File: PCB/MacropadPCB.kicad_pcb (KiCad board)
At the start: 2 copper layers, 38.3 x 79.7 mm, 9 parts, among them SW1 SW_Push, SW2 SW_Push, SW3 SW_Push, SW4 SW_Push, SW5 SW_Push, SW6 SW_Push, U1 XIAO-RP2040-DIP

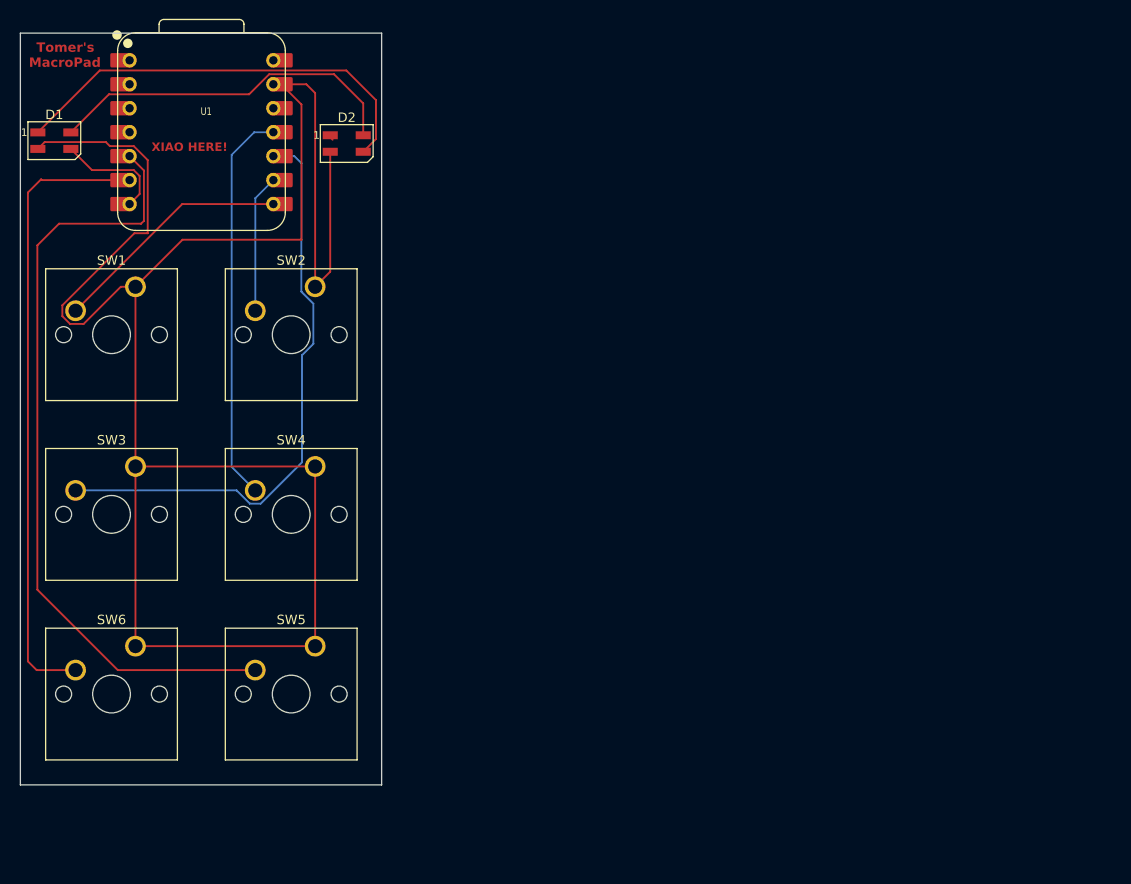
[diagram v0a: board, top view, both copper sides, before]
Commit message: VERSION 3
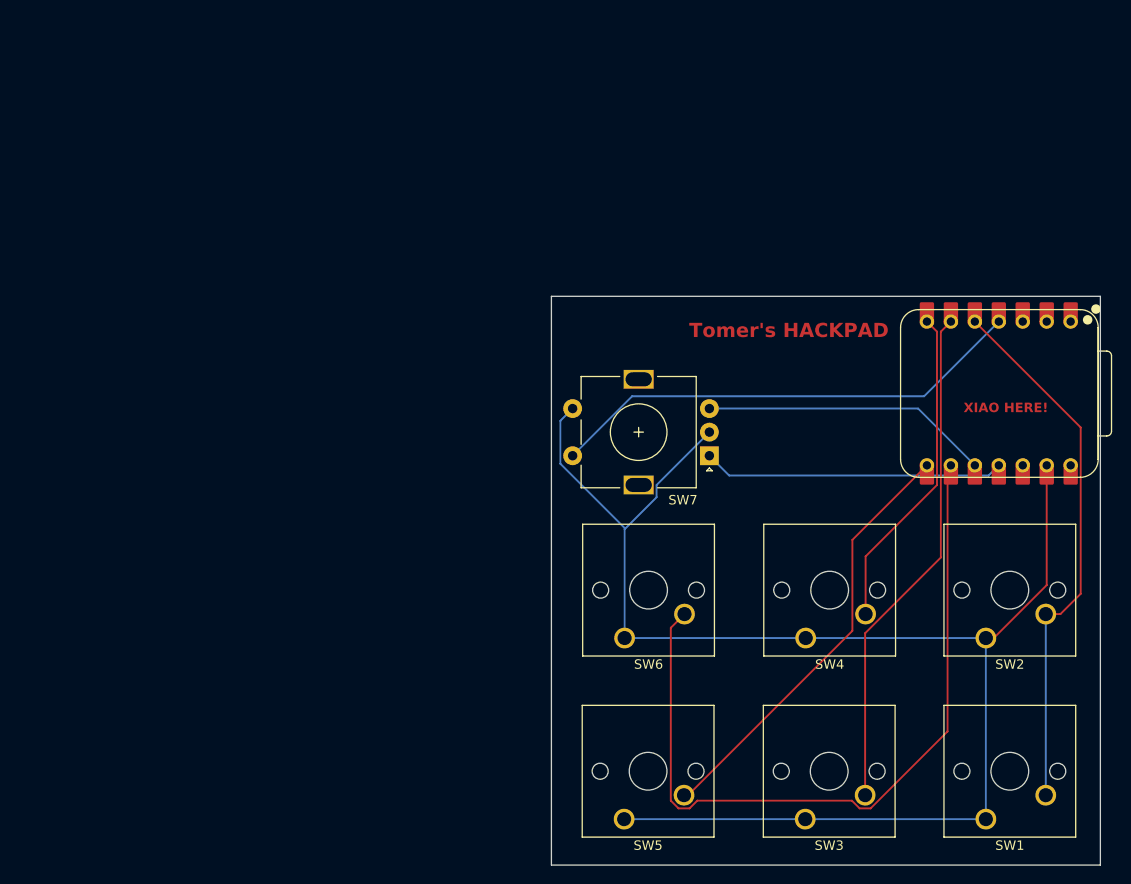
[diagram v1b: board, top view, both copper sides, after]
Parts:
- removed D1, D2: SK6812MINI, LED_SMD:LED_SK6812MINI_PLCC4_3.5x3.5mm_P1.75mm
- added SW7: RotaryEncoder_Switch, Rotary_Encoder:RotaryEncoder_Alps_EC11E-Switch_Vertical_H20mm, F.Cu at (144.3, 105.7)
- moved SW1 106.4 mm to (173.7, 144.2), turned to 180 degrees
- moved U1 89.0 mm to (175.0, 99.1), turned to -90 degrees
- moved SW2 80.3 mm to (173.7, 125.0), turned to 180 degrees
- moved SW3 80.3 mm to (154.5, 144.2), turned to 180 degrees
- moved SW4 55.1 mm to (154.6, 125.0), turned to 180 degrees
- moved SW6 51.9 mm to (135.4, 125.0), turned to 180 degrees
- moved SW5 37.5 mm to (135.3, 144.2), turned to 180 degrees
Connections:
- SW1 pad 2: Net-(U1-GPIO1/RX) -> Net-(U1-GPIO6/SDA)
- SW2 pad 2: Net-(U1-GPIO2/SCK) -> Net-(U1-GPIO6/SDA)
- SW3 pad 2: Net-(U1-GPIO4/MISO) -> Net-(U1-GPIO7/SCL)
- SW4 pad 2: Net-(U1-GPIO3/MOSI) -> Net-(U1-GPIO0/TX)
- SW5 pad 2: Net-(U1-GPIO6/SDA) -> Net-(U1-GPIO1/RX)
- SW6 pad 2: Net-(U1-GPIO7/SCL) -> Net-(U1-GPIO2/SCK)
- U1 pad 4: unconnected-(U1-GPIO29/ADC3/A3-Pad4) -> Net-(U1-GPIO29/ADC3/A3)
- U1 pad 7: Net-(D1-DIN) -> Net-(U1-GPIO0/TX)
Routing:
- net Net-(U1-GPIO2/SCK): track 14.6 -> 82.5 mm
- net GND: track 216.2 -> 158.2 mm
- net Net-(U1-GPIO29/ADC3/A3): track 0.00 -> 51.1 mm
- net Net-(D1-DOUT): track 45.9 -> 0.00 mm
- net Net-(D1-VDD): track 38.2 -> 0.00 mm
- net Net-(U1-GPIO0/TX): track 0.00 -> 34.6 mm
- net Net-(U1-GPIO4/MISO): track 62.4 -> 30.6 mm
- net Net-(U1-GPIO6/SDA): track 83.0 -> 57.3 mm
- net Net-(U1-GPIO1/RX): track 25.7 -> 45.9 mm
- net Net-(D1-DIN): track 11.9 -> 0.00 mm
- net Net-(U1-GPIO7/SCL): track 65.7 -> 54.0 mm
- net Net-(U1-GPIO3/MOSI): track 42.0 -> 32.0 mm
- net unconnected-(D2-DOUT-Pad1): track 0.58 -> 0.00 mm
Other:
- board size 38.3 x 79.7 mm -> 58.2 x 60.3 mm
- board text added: "Tomer's HACKPAD"
- board text removed: "MacroPad"
- board text removed: "Tomer's"
